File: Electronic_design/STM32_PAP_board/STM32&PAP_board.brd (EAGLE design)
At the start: 100 x 80 mm, 21 parts

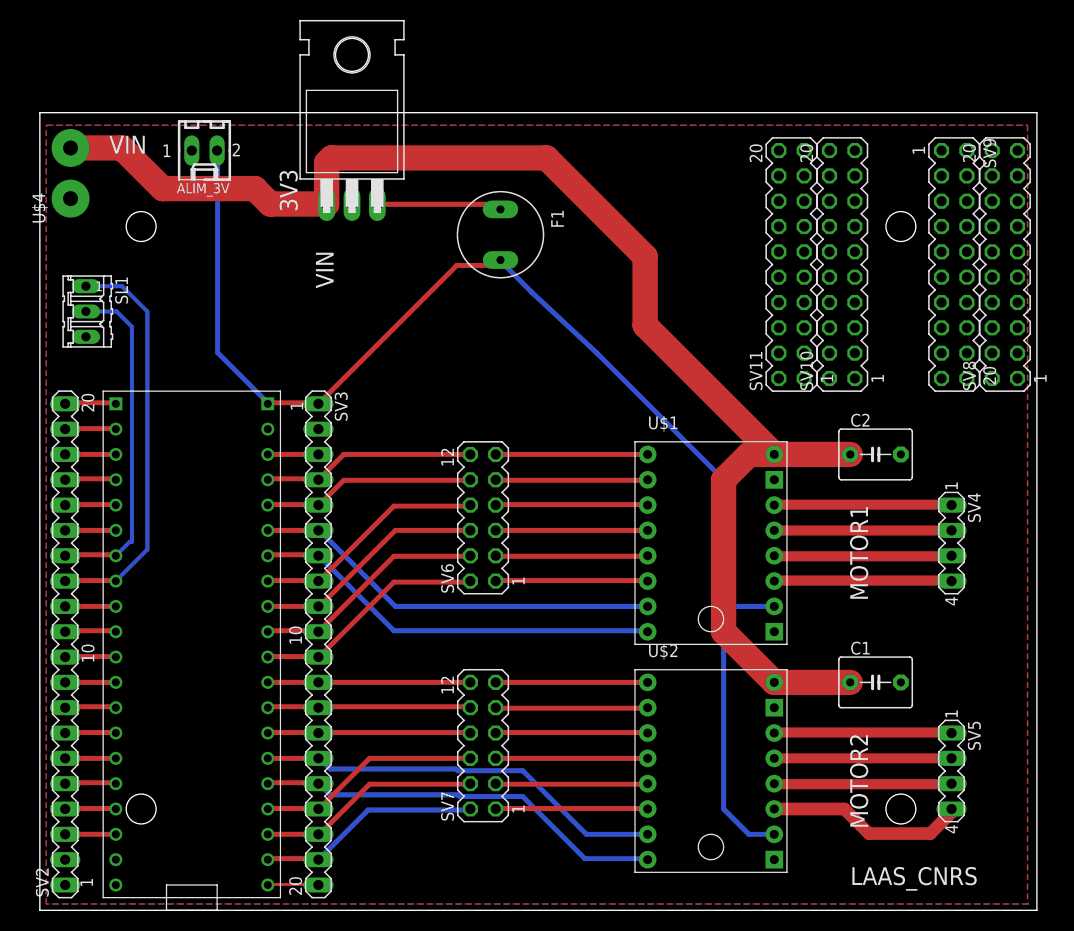
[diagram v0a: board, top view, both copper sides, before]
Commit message: ameliorations
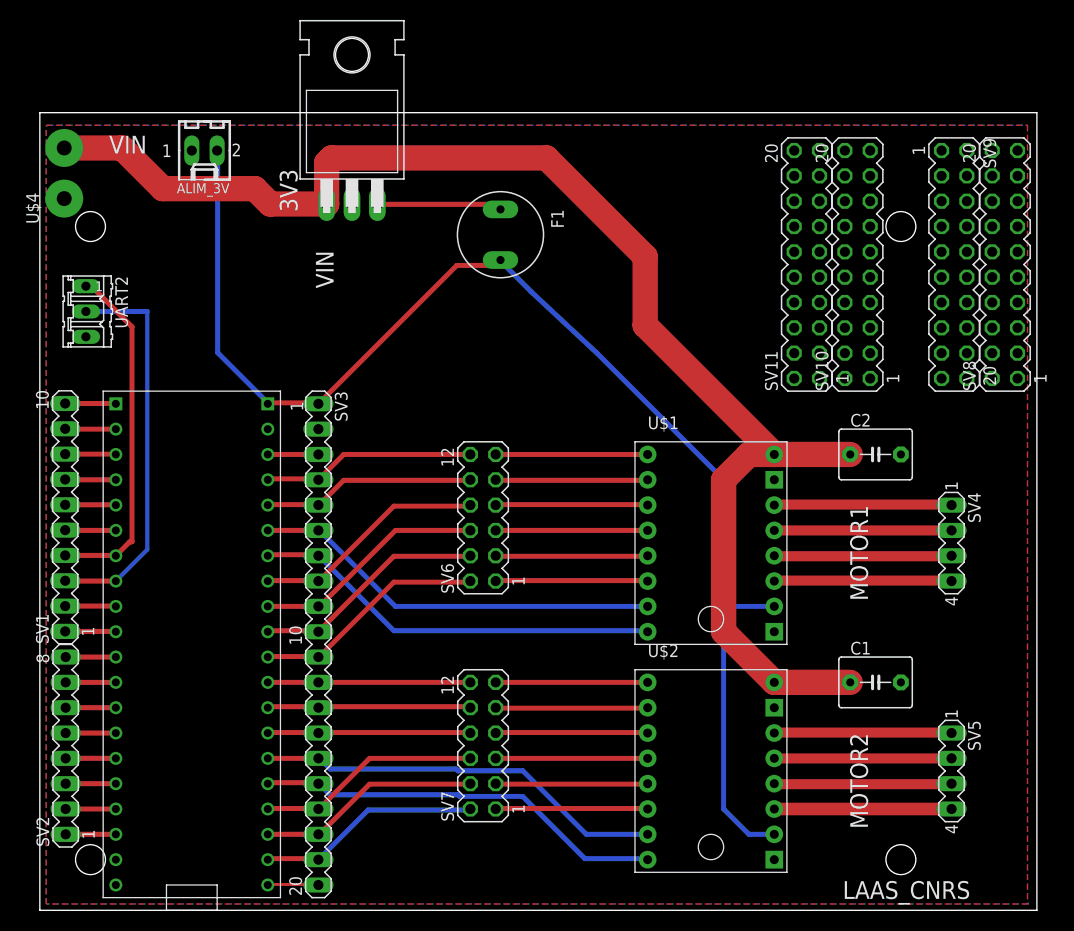
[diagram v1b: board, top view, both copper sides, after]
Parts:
- added SV1: (no value), con-lstb:MA10-1
- SV2: device con-lstb:MA20-1 -> con-lstb:MA08-1
- moved SV2 10.2 mm to (2.59, 16.5)
- moved SV10 1.54 mm to (82.0, 64.8)
- moved SV11 1.54 mm to (76.9, 64.8)
- moved U$4 0.64 mm to (2.44, 73.9)
- renumbered SL1 to UART2
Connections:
- net GND: no longer SV2.1, SV2.2
- net N$10: now also SV2.8; no longer SV2.10
- net N$11: now also SV1.1; no longer SV2.11
- net N$12: now also SV1.2; no longer SV2.12
- net N$13: now also SV1.3, UART2.2; no longer SV2.13, UART2.1
- net N$14: now also SV1.4, UART2.1; no longer SV2.14, UART2.2
- net N$15: now also SV1.5; no longer SV2.15
- net N$16: now also SV1.6; no longer SV2.16
- net N$17: now also SV1.7; no longer SV2.17
- net N$18: now also SV1.8; no longer SV2.18
- net N$19: now also SV1.9; no longer SV2.19
- net N$20: now also SV1.10; no longer SV2.20
- net N$3: now also SV2.1; no longer SV2.3
- net N$4: now also SV2.2; no longer SV2.4
- net N$5: now also SV2.3; no longer SV2.5
- net N$6: now also SV2.4; no longer SV2.6
- net N$7: now also SV2.5; no longer SV2.7
- net N$8: now also SV2.6; no longer SV2.8
- net N$9: now also SV2.7; no longer SV2.9
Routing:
- net N$44: track 20.2 -> 17.9 mm
- net N$13: track 40.7 -> 39.7 mm
- net N$14: track 34.3 -> 35.3 mm
- net N$42: track 137.4 -> 138.1 mm
- net GND: track 0.61 -> 0.00 mm
